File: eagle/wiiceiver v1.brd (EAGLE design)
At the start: 100 x 80 mm, 15 parts, among them IC1 ATmega328P, IC2 317T

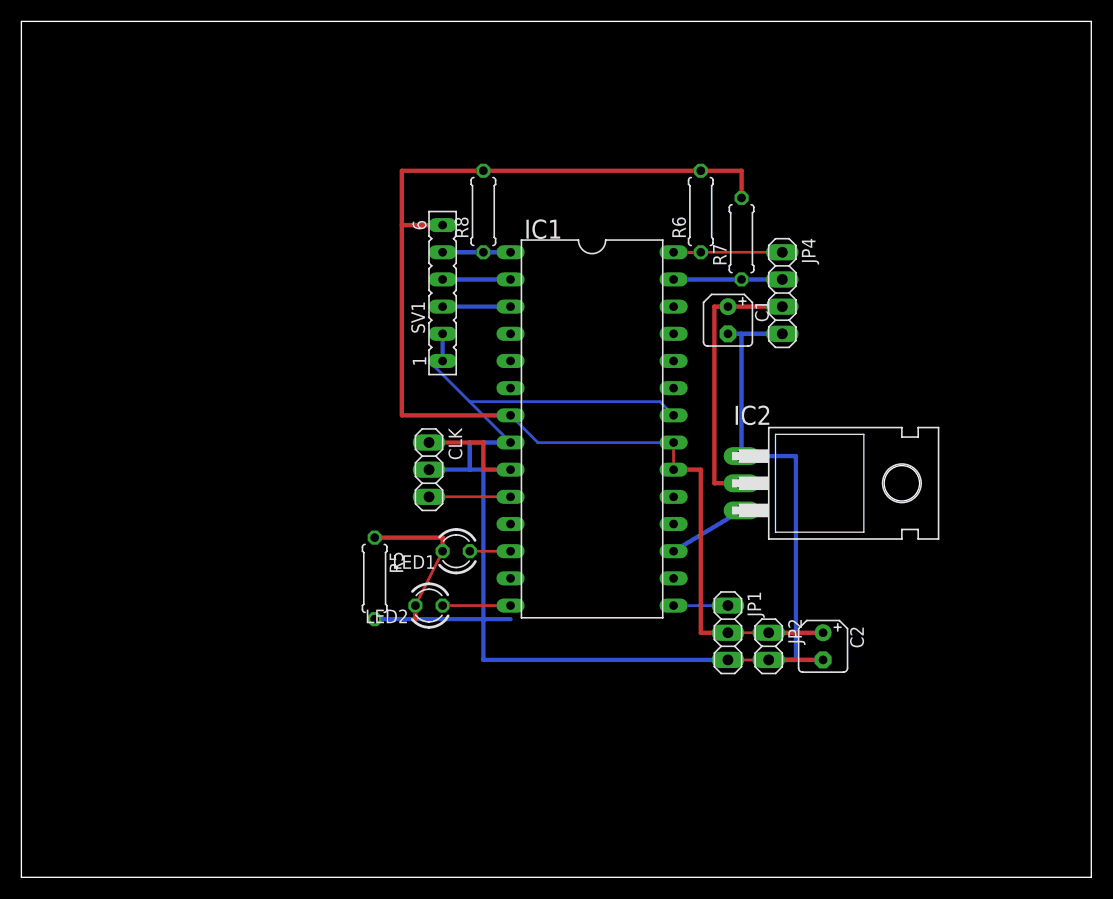
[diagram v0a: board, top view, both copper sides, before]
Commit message: ordered!
“final” version, ordered from OshPark
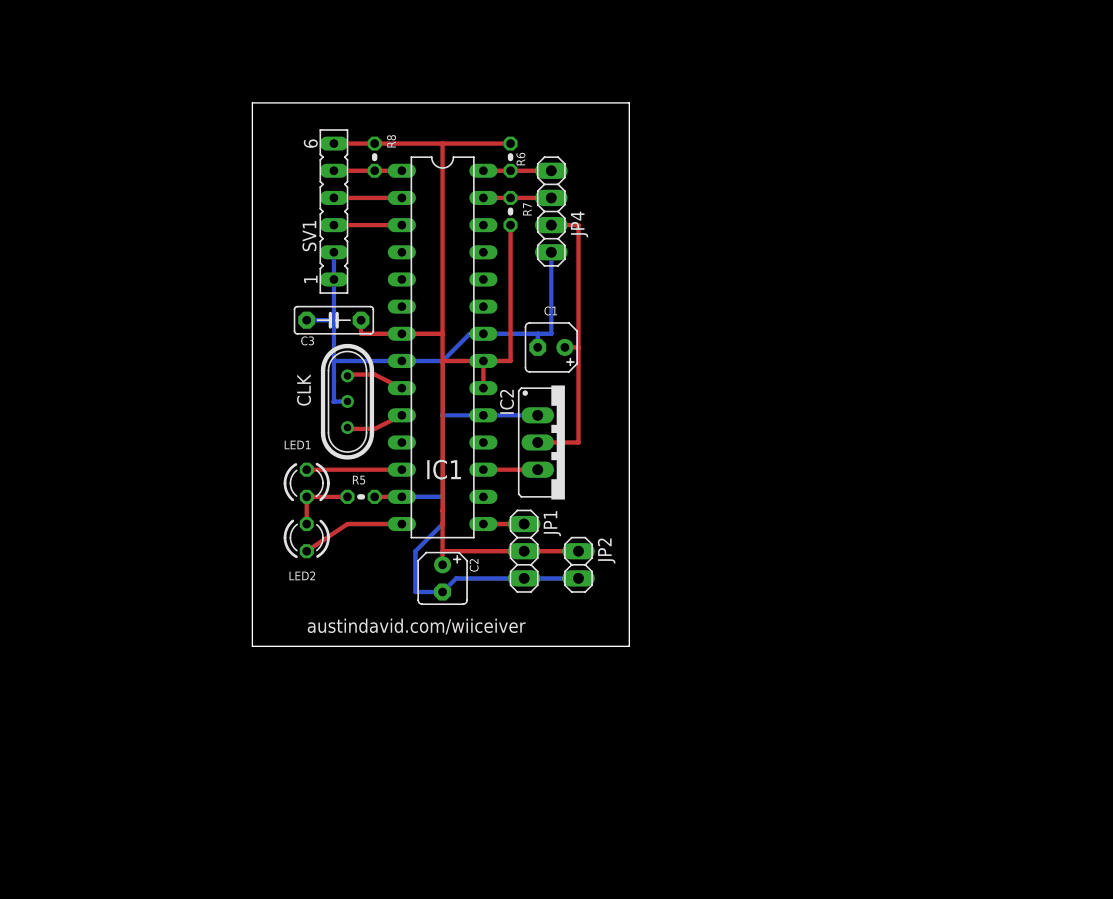
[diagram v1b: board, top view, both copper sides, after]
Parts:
- added C3: 0.1pF, capacitor-wima:C5B2.5
- CLK: device pinhead:1X03 -> crystal:HC49U
- IC1: device ic-package:DIL28-6 -> ic-package:DIL28-3
- IC2: value 317T -> (none); device linear:TO220H -> v-reg:317TS
- R5, R6, R7, R8: device rcl:0207/7 -> resistor:0204V
- moved C2 36.1 mm to (39.4, 27.9)
- moved IC2 26.9 mm to (50.8, 40.6)
- moved JP4 22.9 mm to (49.5, 62.2)
- moved R7 21.7 mm to (45.7, 62.2), turned to 270 degrees
- moved JP1 20.5 mm to (47.0, 30.5)
- moved JP2 19.3 mm to (52.1, 29.2)
- moved R6 18.5 mm to (45.7, 67.3)
- moved C1 16.7 mm to (49.5, 49.5), turned to 180 degrees
- moved IC1 15.9 mm to (39.4, 49.5)
- moved LED1 15.3 mm to (26.7, 36.8), turned to 270 degrees
- moved LED2 13.1 mm to (26.7, 31.8), turned to 90 degrees
- moved SV1 12.7 mm to (29.2, 62.2)
- moved R8 11.4 mm to (33.0, 67.3), turned to 270 degrees
- moved CLK 9.92 mm to (30.5, 44.5)
- moved R5 7.73 mm to (31.8, 35.6), turned to 0 degrees
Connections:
- removed net N$12: IC1.1, R8.1, SV1.5
- new net N$2: IC1.1, R8.2, SV1.5
- net GND: now also C3.2
- net VIN: now also C3.1, R8.1; no longer R8.2
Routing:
- net GND: track 151.0 -> 101.7 mm
- net VIN: track 119.2 -> 99.1 mm
- net N$6: track 14.6 -> 6.35 mm
- net N$21: track 12.7 -> 6.35 mm
- net N$2: track 0.00 -> 6.35 mm
- net N$12: track 6.35 -> 0.00 mm
- net DIP12: track 3.81 -> 8.89 mm
- net N$11: track 10.2 -> 5.38 mm
- net N$22: track 10.2 -> 6.35 mm
- net N$7: track 6.35 -> 9.66 mm
- net N$16: track 25.4 -> 27.9 mm
- net N$10: track 7.41 -> 5.08 mm
- net N$9: track 7.62 -> 5.38 mm
- net N$1: track 5.08 -> 3.81 mm
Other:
- board size 100 x 80 mm -> 35.2 x 50.8 mm
- board text added: "austindavid.com/wiiceiver"
